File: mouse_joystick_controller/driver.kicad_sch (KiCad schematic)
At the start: 13 parts, among them J1 Conn_FFC_20_Pin_1mm_bottom-ZF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, U1 LVDS_4-4_HALF_DS91M040TSQE, U2 LVDS_4-4_HALF_DS91M040TSQE

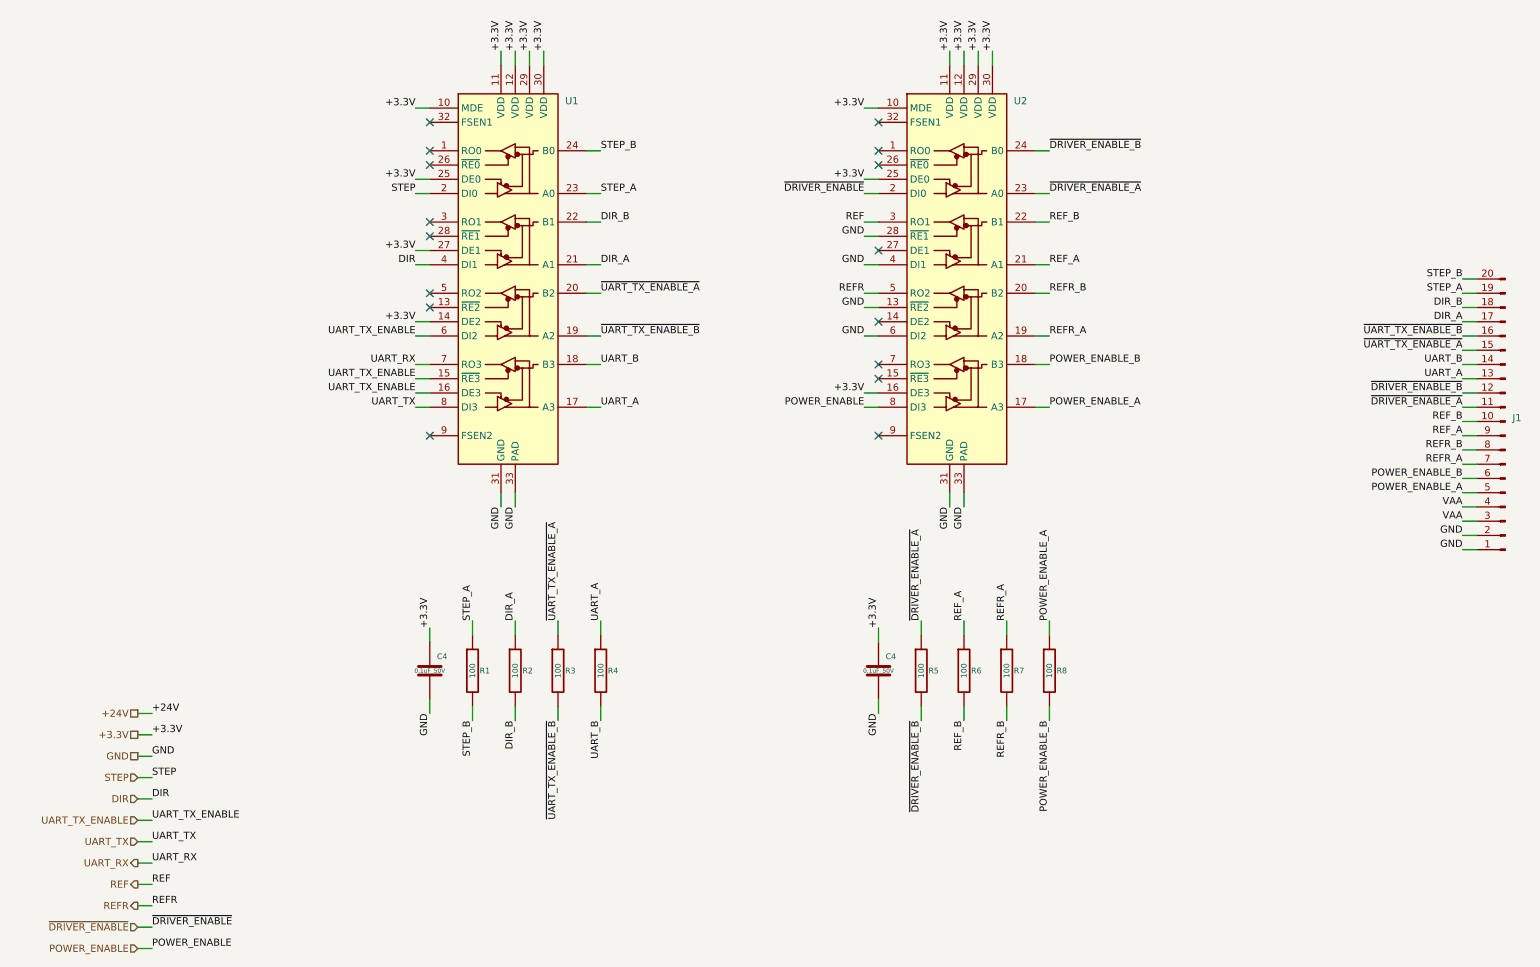
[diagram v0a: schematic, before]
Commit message: Add power jack
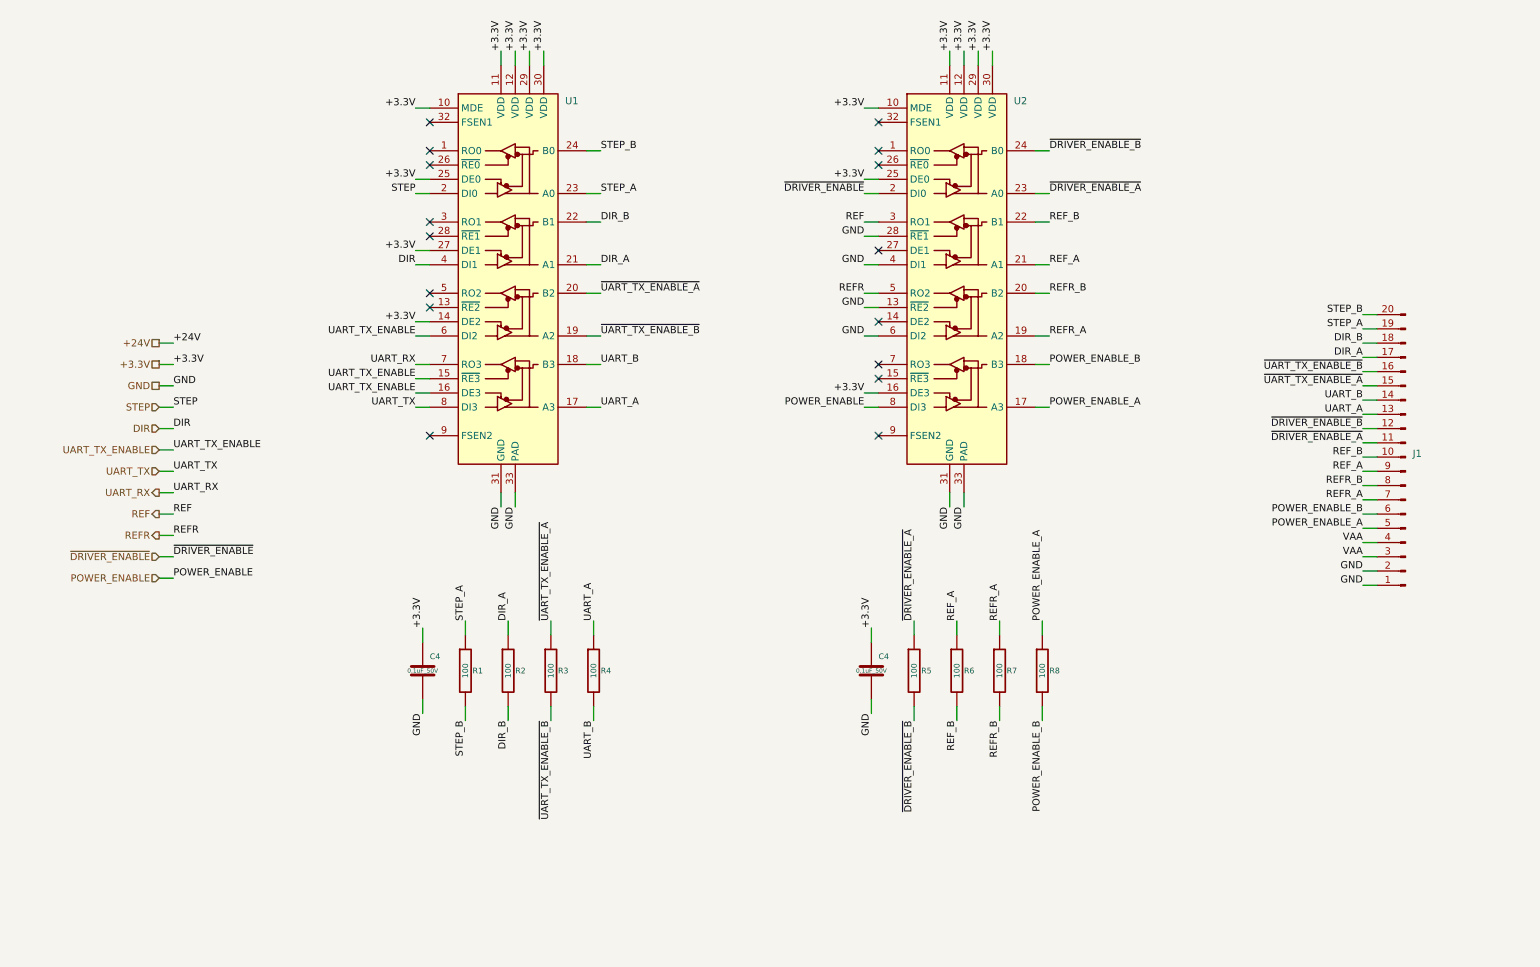
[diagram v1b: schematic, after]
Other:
- moved on the sheet: C4, J1, R1, R2, R3, R4, R5, R6, R7, R8
